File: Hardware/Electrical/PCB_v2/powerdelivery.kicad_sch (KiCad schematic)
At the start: 27 parts, among them J2 USB_C_Receptacle_USB2.0_16P, Q1 Q_PMOS, Q2 Q_PMOS, Q3 Q_PMOS, Q4 Q_PMOS, U2 TPD2EUSB30, U3 CYPD3177-24LQ

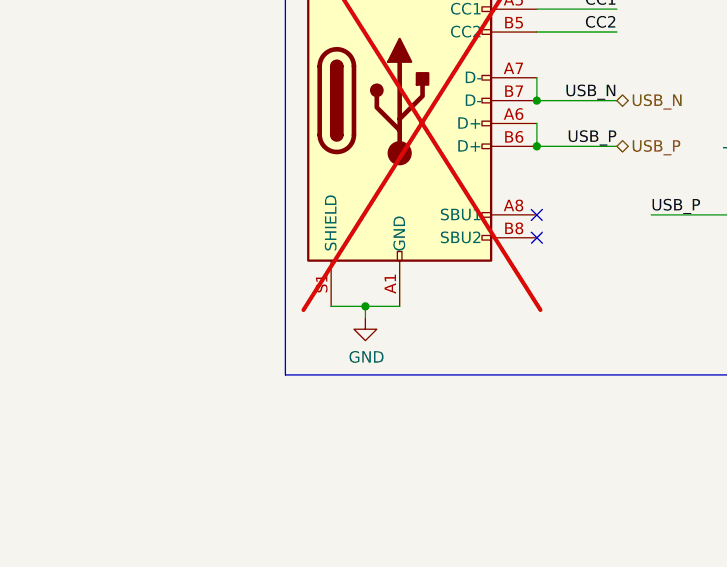
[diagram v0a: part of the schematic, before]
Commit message: PCB finished, export working
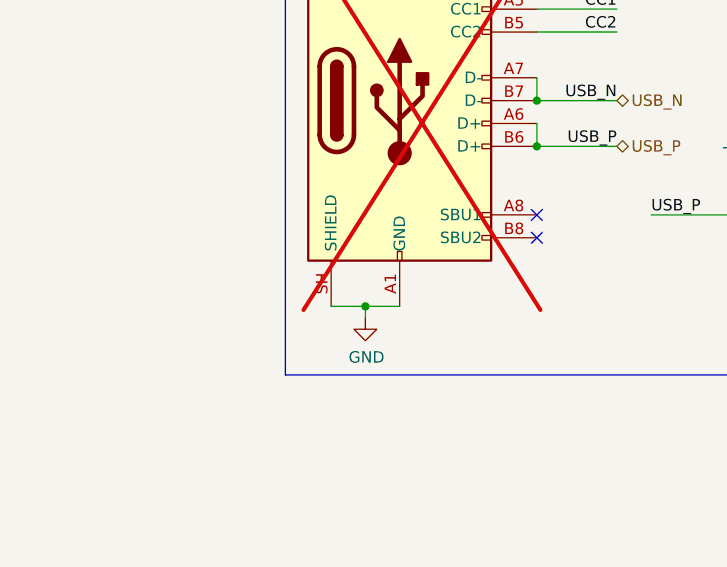
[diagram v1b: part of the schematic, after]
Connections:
- net GND: now also J2.SH (SHIELD); no longer J2.S1 (SHIELD)
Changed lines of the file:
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@@
+			)
+		)
+		(property "Manufacturer" ""
+			(at 73.66 87.63 0)
+			(hide yes)
+			(show_name no)
+			(do_not_autoplace no)
+			(effects
+				(font
+					(size 1.27 1.27)
+				)
 			)
 		)
@@
 		(pin "B9"
 		)
-		(pin "S1"
+		(pin "SH"
 		)
 		(pin "A5"
